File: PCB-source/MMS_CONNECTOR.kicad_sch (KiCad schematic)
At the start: 6 parts, among them J9 RJ45_LED_Shielded, U3 TPD2EUSB30DRTR-TP

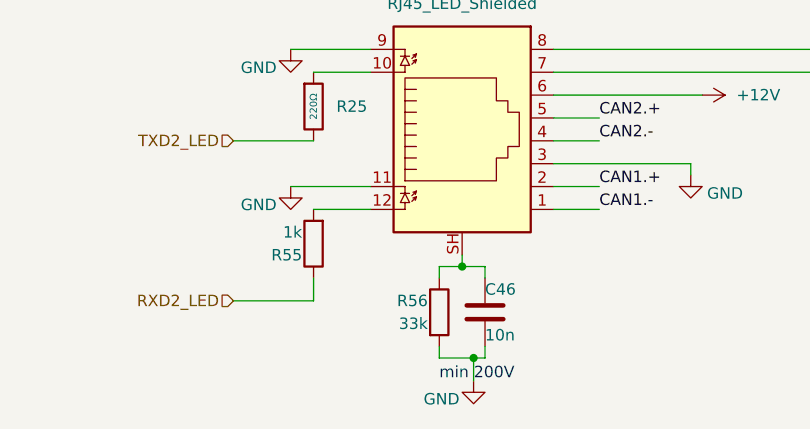
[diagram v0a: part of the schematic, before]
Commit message: bom done
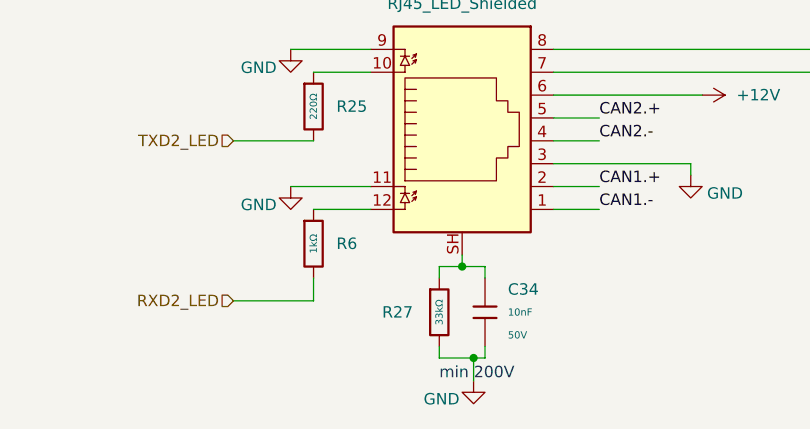
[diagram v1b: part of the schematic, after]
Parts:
- removed C46: 10n, Capacitor_SMD:C_0402_1005Metric, symbol Device:C
- removed R55: 1k, Resistor_SMD:R_0402_1005Metric, symbol Device:R
- removed R56: 33k, Resistor_SMD:R_0402_1005Metric, symbol Device:R
- added C34: 10nF, PCM_JLCPCB:C_0402, symbol PCM_JLCPCB-Capacitors:0402,10nF
- added R27: 33kΩ, PCM_JLCPCB:R_0402, symbol PCM_JLCPCB-Resistors:0402,33kΩ
- added R6: 1kΩ, PCM_JLCPCB:R_0402, symbol PCM_JLCPCB-Resistors:0402,1kΩ
- J9: now left out of the parts list
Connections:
- net GND: now also C34.2, R27.2
- net RXD2_LED: now also R6.2
- net at J9.12: now also R6.1
- net at J9.SH: now also C34.1, R27.1

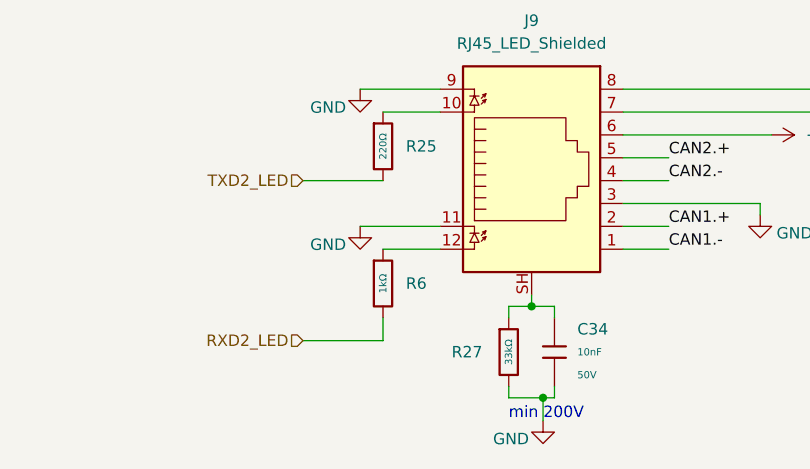
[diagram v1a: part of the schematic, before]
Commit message: REV A production ready
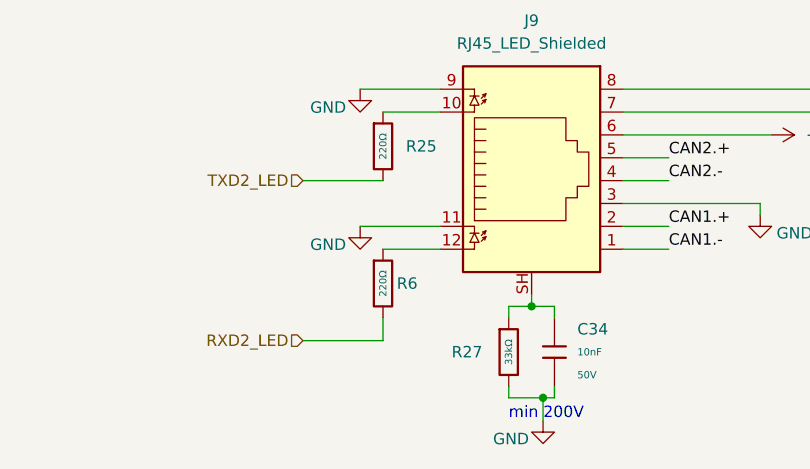
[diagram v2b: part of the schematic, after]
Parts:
- removed R6: 1kΩ, PCM_JLCPCB:R_0402, symbol PCM_JLCPCB-Resistors:0402,1kΩ
- added R6: 220Ω, PCM_JLCPCB:R_0402, symbol PCM_JLCPCB-Resistors:0402,220Ω
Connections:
- net RXD2_LED: now also R6.2
- net at J9.12: now also R6.1
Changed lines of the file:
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@@
+	)
+	(symbol
+		(lib_id "PCM_JLCPCB-Resistors:0402,220Ω")
+		(at 113.03 107.95 0)
+		(unit 1)
+		(exclude_from_sim no)
+		(in_bom yes)
+		(on_board yes)
+		(dnp no)
+		(property "Reference" "R6"
+			(at 114.554 107.95 0)
+			(effects
+				(font
+					(size 1.27 1.27)
+				)
+				(justify left)
+			)
+		)
+		(property "Value" "220Ω"
+			(at 113.03 107.95 90)
+			(do_not_autoplace yes)
+			(effects
+				(font
+					(size 0.8 0.8)
+				)
+			)
+		)
+		(property "Footprint" "PCM_JLCPCB:R_0402"
+			(at 111.252 107.95 90)
+			(effects
+				(font
+					(size 1.27 1.27)
+				)
+				(hide yes)
+			)
+		)
+		(property "Datasheet" "https://www.lcsc.com/datasheet/lcsc_datasheet_2205311900_UNI-ROYAL-Uniroyal-Elec-0402WGF2200TCE_C25091.pdf"
+			(at 113.03 107.95 0)
+			(effects
+				(font
+					(size 1.27 1.27)
+				)
+				(hide yes)
+			)
+		)
+		(property "Description" "62.5mW Thick Film Resistors 50V ±100ppm/°C ±1% 220Ω 0402 Chip Resistor - Surface Mount ROHS"
+			(at 113.03 107.95 0)
+			(effects
+				(font
+					(size 1.27 1.27)
+				)
+				(hide yes)
+			)
+		)
+		(property "LCSC" "C25091"
+			(at 113.03 107.95 0)
+			(effects
+				(font
+					(size 1.27 1.27)
+				)
+				(hide yes)
+			)
+		)
+		(property "Stock" "617243"
+			(at 113.03 107.95 0)
+			(effects
+				(font
+					(size 1.27 1.27)
+				)
+				(hide yes)
+			)
+		)
+		(property "Price" "0.004USD"
+			(at 113.03 107.95 0)
+			(effects
+				(font
+					(size 1.27 1.27)
+				)
+				(hide yes)
+			)
+		)
+		(property "Process" "SMT"
+			(at 113.03 107.95 0)
+			(effects
+				(font
+					(size 1.27 1.27)
+				)
+				(hide yes)
+			)
+		)
+		(property "Minimum Qty" "20"
+			(at 113.03 107.95 0)
+			(effects
+				(font
+					(size 1.27 1.27)
+				)
+				(hide yes)
+			)
+		)
+		(property "Attrition Qty" "10"
+			(at 113.03 107.95 0)
+			(effects
+				(font
+					(size 1.27 1.27)
+				)
+				(hide yes)
+			)
+		)
+		(property "Class" "Basic Component"
+			(at 113.03 107.95 0)
+			(effects
+				(font
+					(size 1.27 1.27)
+				)
+				(hide yes)
+			)
+		)
+		(property "Category" "Resistors,Chip Resistor - Surface Mount"
+			(at 113.03 107.95 0)
+			(effects
+				(font
+					(size 1.27 1.27)
+				)
+				(hide yes)
+			)
+		)
+		(property "Manufacturer" "UNI-ROYAL(Uniroyal Elec)"
+			(at 113.03 107.95 0)
+			(effects
+				(font
+					(size 1.27 1.27)
+				)
+				(hide yes)
+			)
+		)
+		(property "Part" "0402WGF2200TCE"
+			(at 113.03 107.95 0)
+			(effects
+				(font
+					(size 1.27 1.27)
+				)
+				(hide yes)
+			)
+		)
+		(property "Resistance" "220Ω"
+			(at 113.03 107.95 0)
+			(effects
+				(font
+					(size 1.27 1.27)
+				)
+				(hide yes)
+			)
+		)
+		(property "Power(Watts)" "62.5mW"
+			(at 113.03 107.95 0)
+			(effects
+				(font
+					(size 1.27 1.27)
+				)
+				(hide yes)
+			)
+		)
+		(property "Type" "Thick Film Resistors"
+			(at 113.03 107.95 0)
+			(effects
+				(font
+					(size 1.27 1.27)
+				)
+				(hide yes)
+			)
+		)
+		(property "Overload Voltage (Max)" "50V"
+			(at 113.03 107.95 0)
+			(effects
+				(font
+					(size 1.27 1.27)
+				)
+				(hide yes)
+			)
+		)
+		(property "Operating Temperature Range" "-55°C~+155°C"
+			(at 113.03 107.95 0)
+			(effects
+				(font
+					(size 1.27 1.27)
+				)
+				(hide yes)
+			)
+		)
+		(property "Tolerance" "±1%"
+			(at 113.03 107.95 0)
+			(effects
+				(font
+					(size 1.27 1.27)
+				)
+				(hide yes)
+			)
+		)
+		(property "Temperature Coefficient" "±100ppm/°C"
+			(at 113.03 107.95 0)
+			(effects
+				(font
+					(size 1.27 1.27)
+				)
+				(hide yes)
+			)
+		)
+		(pin "1"
+		)
+		(pin "2"
+		)
+		(instances
+			(project "MMS2"
+				(path "/6596548a-44e0-46d8-8624-fd71cf4a3e17/375a4799-1237-4cf9-80bd-b6d6bc52fffa"
+					(reference "R53")
+					(unit 1)
+				)
+				(path "/6596548a-44e0-46d8-8624-fd71cf4a3e17/6dbf7263-2614-4625-a960-703f6ff0d778"
+					(reference "R6")
+					(unit 1)
+				)
+			)
+		)
 	)
 	(symbol
@@
 					(unit 1)
 				)
-			)
-		)
-	)
-	(symbol
-		(lib_id "PCM_JLCPCB-Resistors:0402,1kΩ")
-		(at 113.03 107.95 0)
-		(unit 1)
-		(exclude_from_sim no)
-		(in_bom yes)
-		(on_board yes)
-		(dnp no)
-		(fields_autoplaced yes)
-		(property "Reference" "R6"
-			(at 115.57 107.9499 0)
-			(effects
-				(font
-					(size 1.27 1.27)
-				)
-				(justify left)
-			)
-		)
-		(property "Value" "1kΩ"
-			(at 113.03 107.95 90)
-			(do_not_autoplace yes)
-			(effects
-				(font
-					(size 0.8 0.8)
-				)
-			)
-		)
-		(property "Footprint" "PCM_JLCPCB:R_0402"
-			(at 111.252 107.95 90)
-			(effects
-				(font
-					(size 1.27 1.27)
-				)
-				(hide yes)
-			)
-		)
-		(property "Datasheet" "https://www.lcsc.com/datasheet/lcsc_datasheet_2206010216_UNI-ROYAL-Uniroyal-Elec-0402WGF1001TCE_C11702.pdf"
-			(at 113.03 107.95 0)
-			(effects
-				(font
-					(size 1.27 1.27)
-				)
-				(hide yes)
-			)
-		)
-		(property "Description" "62.5mW Thick Film Resistors 50V ±100ppm/°C ±1% 1kΩ 0402 Chip Resistor - Surface Mount ROHS"
-			(at 113.03 107.95 0)
-			(effects
-				(font
-					(size 1.27 1.27)
-				)
-				(hide yes)
-			)
-		)
-		(property "LCSC" "C11702"
-			(at 113.03 107.95 0)
-			(effects
-				(font
-					(size 1.27 1.27)
-				)
-				(hide yes)
-			)
-		)
-		(property "Stock" "6889074"
-			(at 113.03 107.95 0)
-			(effects
-				(font
-					(size 1.27 1.27)
-				)
-				(hide yes)
-			)
-		)
-		(property "Price" "0.004USD"
-			(at 113.03 107.95 0)
-			(effects
-				(font
-					(size 1.27 1.27)
-				)
-				(hide yes)
-			)
-		)
-		(property "Process" "SMT"
-			(at 113.03 107.95 0)
-			(effects
-				(font
-					(size 1.27 1.27)
-				)
-				(hide yes)
-			)
-		)
-		(property "Minimum Qty" "20"
-			(at 113.03 107.95 0)
-			(effects
-				(font
-					(size 1.27 1.27)
-				)
-				(hide yes)
-			)
-		)
-		(property "Attrition Qty" "10"
-			(at 113.03 107.95 0)
-			(effects
-				(font
-					(size 1.27 1.27)
-				)
-				(hide yes)
-			)
-		)
-		(property "Class" "Basic Component"
-			(at 113.03 107.95 0)
-			(effects
-				(font
-					(size 1.27 1.27)
-				)
-				(hide yes)
-			)
-		)
-		(property "Category" "Resistors,Chip Resistor - Surface Mount"
-			(at 113.03 107.95 0)
-			(effects
-				(font
-					(size 1.27 1.27)
-				)
-				(hide yes)
-			)
-		)
-		(property "Manufacturer" "UNI-ROYAL(Uniroyal Elec)"
-			(at 113.03 107.95 0)
-			(effects
-				(font
-					(size 1.27 1.27)
-				)
-				(hide yes)
-			)
-		)
-		(property "Part" "0402WGF1001TCE"
-			(at 113.03 107.95 0)
-			(effects
-				(font
-					(size 1.27 1.27)
-				)
-				(hide yes)
-			)
-		)
-		(property "Resistance" "1kΩ"
-			(at 113.03 107.95 0)
-			(effects
-				(font
-					(size 1.27 1.27)
-				)
-				(hide yes)
-			)
-		)
-		(property "Power(Watts)" "62.5mW"
-			(at 113.03 107.95 0)
-			(effects
-				(font
-					(size 1.27 1.27)
-				)
-				(hide yes)
-			)
-		)
-		(property "Type" "Thick Film Resistors"
-			(at 113.03 107.95 0)
-			(effects
-				(font
-					(size 1.27 1.27)
-				)
-				(hide yes)
-			)
-		)
-		(property "Overload Voltage (Max)" "50V"
-			(at 113.03 107.95 0)
-			(effects
-				(font
-					(size 1.27 1.27)
-				)
-				(hide yes)
-			)
-		)
-		(property "Operating Temperature Range" "-55°C~+155°C"
-			(at 113.03 107.95 0)
-			(effects
-				(font
-					(size 1.27 1.27)
-				)
-				(hide yes)
-			)
-		)
-		(property "Tolerance" "±1%"
-			(at 113.03 107.95 0)
-			(effects
-				(font
-					(size 1.27 1.27)
-				)
-				(hide yes)
-			)
-		)
-		(property "Temperature Coefficient" "±100ppm/°C"
-			(at 113.03 107.95 0)
-			(effects
-				(font
-					(size 1.27 1.27)
-				)
-				(hide yes)
-			)
-		)
-		(pin "2"
-		)
-		(pin "1"
-		)
-		(instances
-			(project ""
-				(path "/6596548a-44e0-46d8-8624-fd71cf4a3e17/375a4799-1237-4cf9-80bd-b6d6bc52fffa"
-					(reference "R53")
-					(unit 1)
-				)
-				(path "/6596548a-44e0-46d8-8624-fd71cf4a3e17/6dbf7263-2614-4625-a960-703f6ff0d778"
-					(reference "R6")
-					(unit 1)
-				)
